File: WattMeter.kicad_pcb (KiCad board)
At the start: 2 copper layers, 40.8 x 50.2 mm, 27 parts, among them J1 ARM_SWD, P1 CONN_01X02, P2 CONN_01X02, P3 CONN_01X03, P4 CONN_01X04, P5 CONN_01X04, U1 MAQ5283, U2 ACS711, U3 MCP9700, U4 MCP6002, U5 SAMD20E15A-A

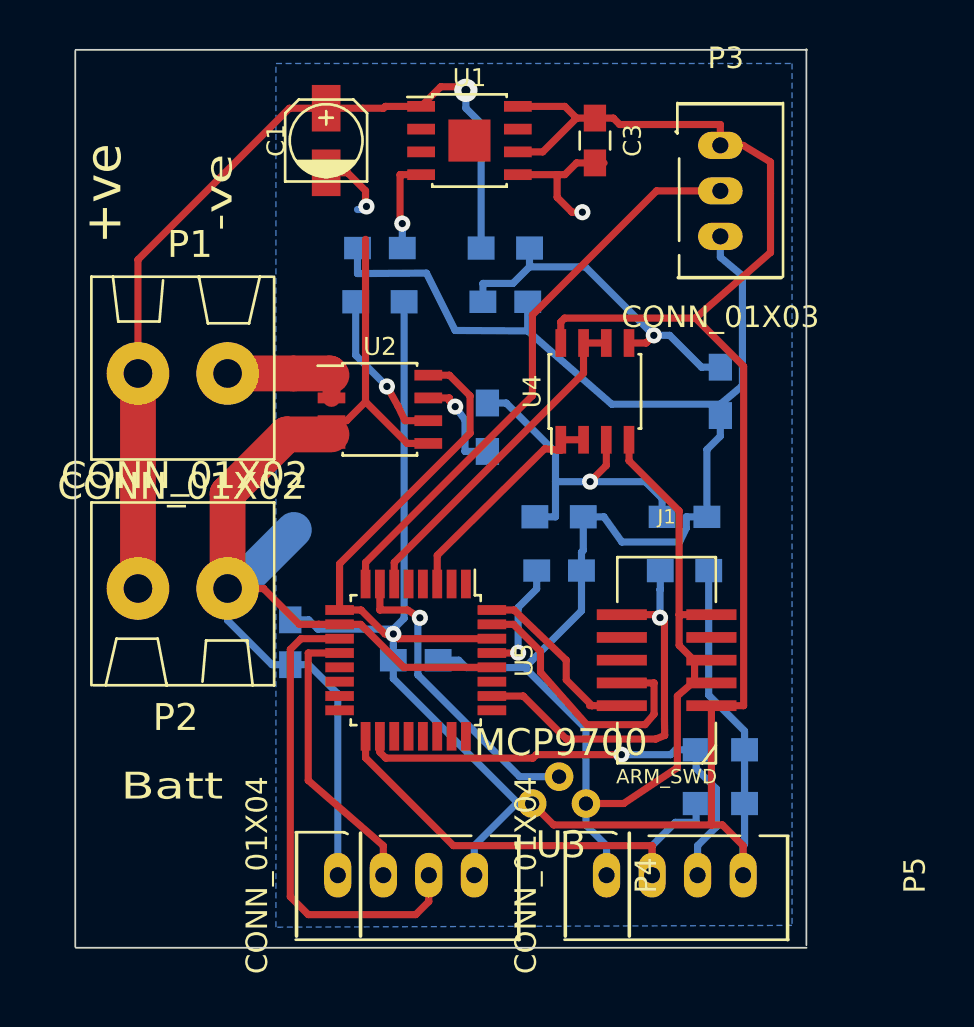
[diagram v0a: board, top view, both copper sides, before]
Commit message: Parts
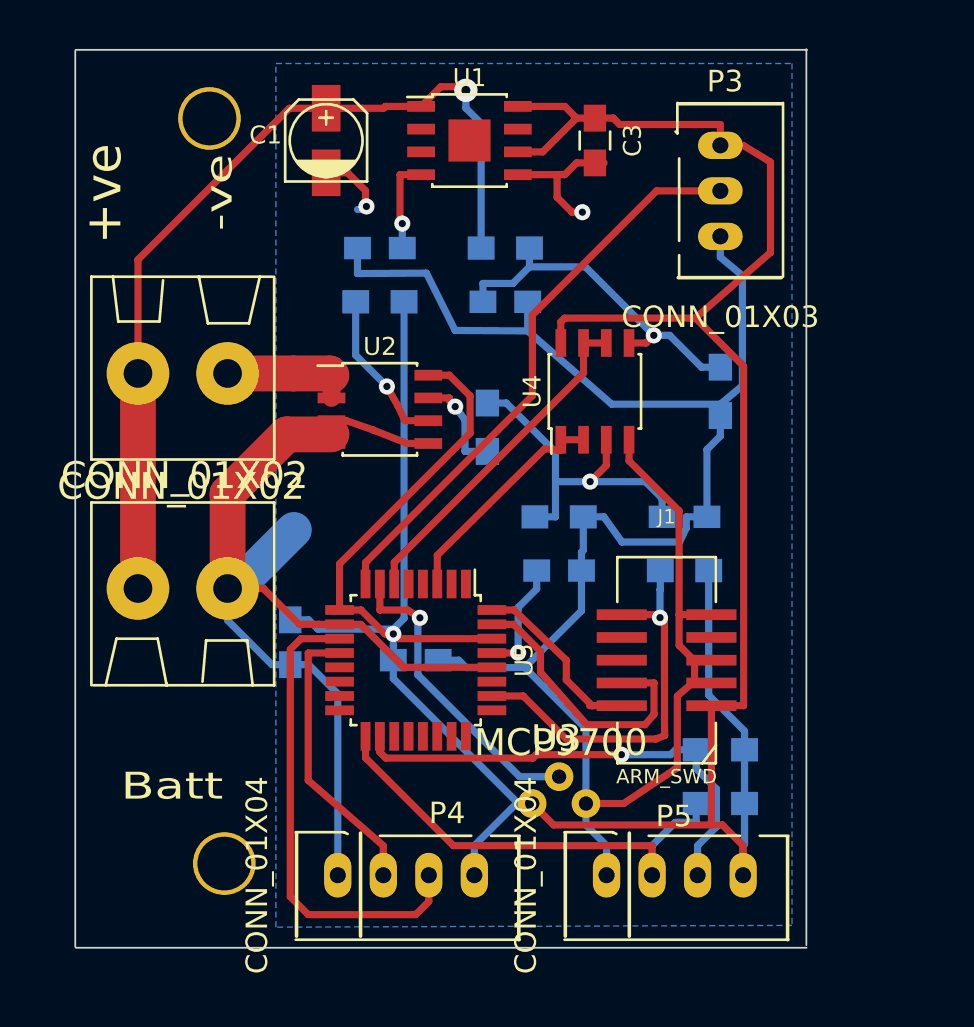
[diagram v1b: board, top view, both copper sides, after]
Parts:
- added 3mm: VAL**, My_Pin_Headers:3mm_mount, F.Cu at (130.5, 83.8)
- added 3mm: VAL**, My_Pin_Headers:3mm_mount, F.Cu at (131.3, 125.3)
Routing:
- net GND: track 195.8 -> 185.6 mm
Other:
- board text added: "Wattmeter 1.0"
